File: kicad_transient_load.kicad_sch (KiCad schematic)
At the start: 6 parts, among them J1 BNC In, J2 Screw_Terminal_01x02, J3 Conn_02x03_Odd_Even

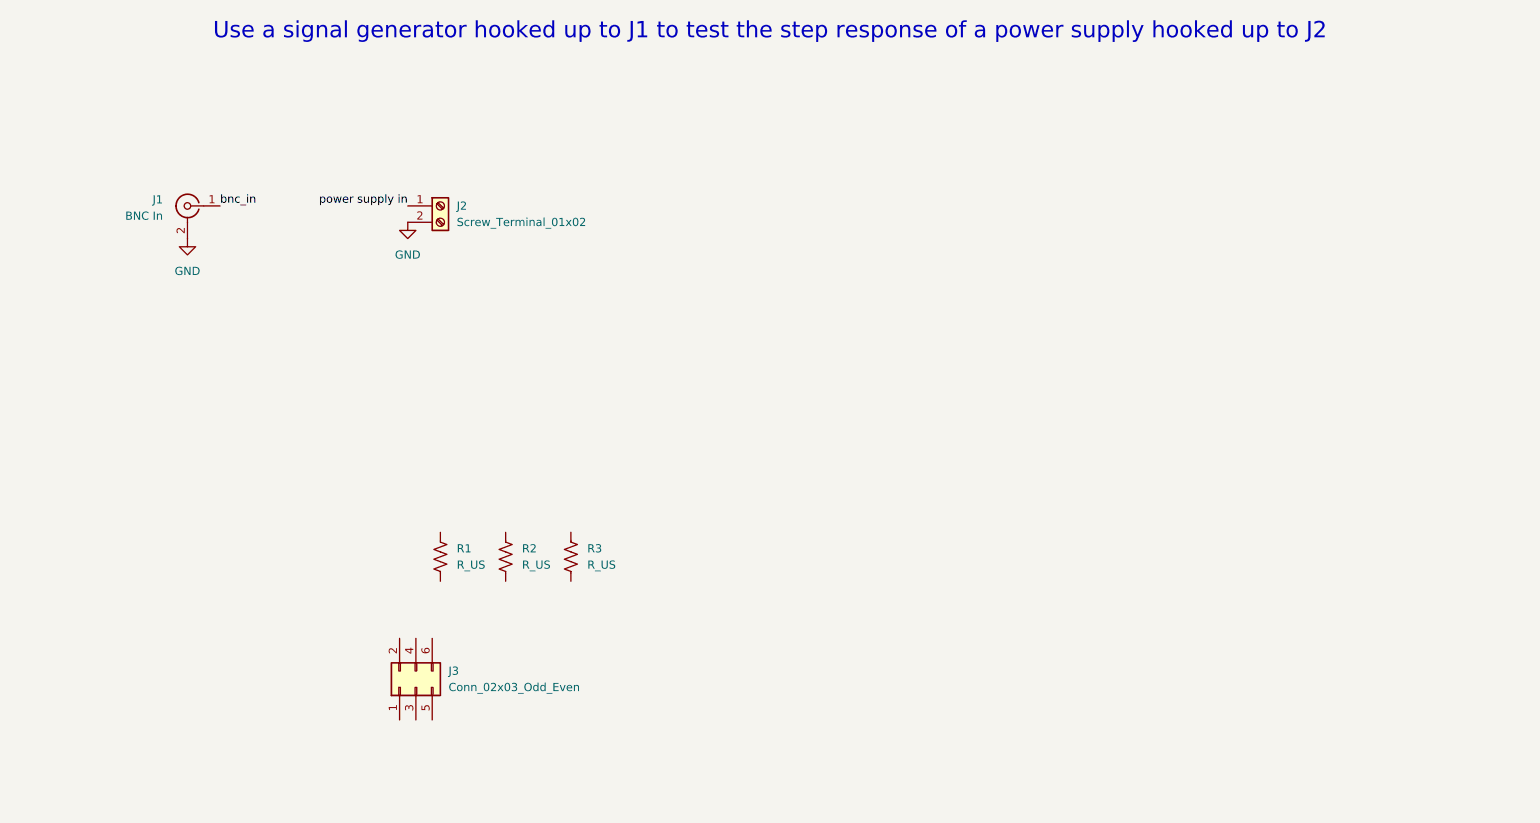
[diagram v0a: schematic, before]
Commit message: schematic laid out
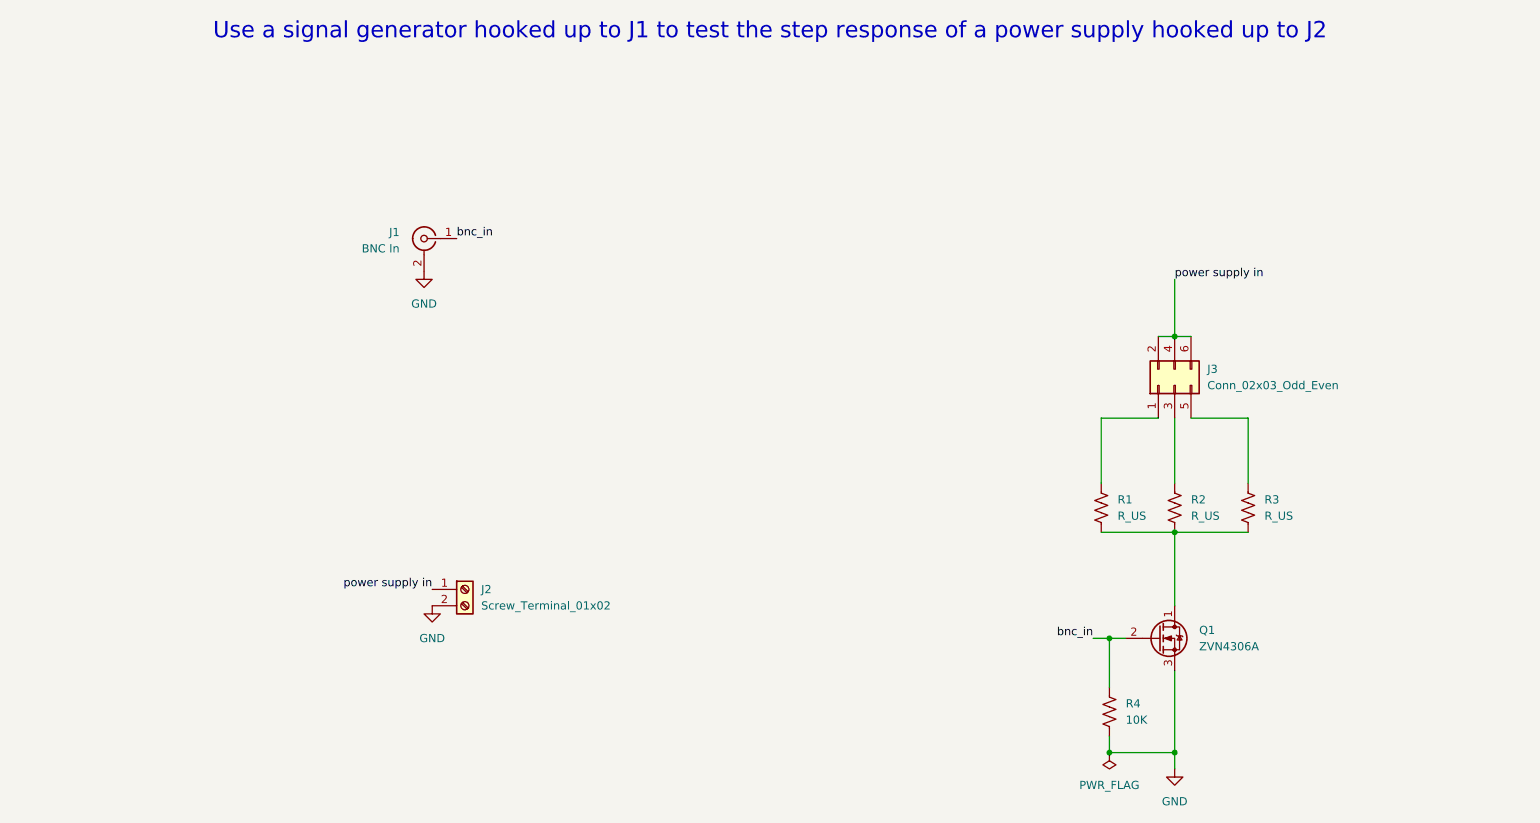
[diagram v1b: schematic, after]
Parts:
- added Q1: ZVN4306A, Package_TO_SOT_THT:TO-92_Inline, symbol Device:Q_NMOS_DGS
- added R4: 10K, symbol Device:R_US
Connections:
- net GND: now also Q1.3 (S), R4.1
- net bnc_in: now also Q1.2 (G), R4.2
- net power supply in: now also J3.2 (Pin_2), J3.4 (Pin_4), J3.6 (Pin_6)
- net at R3.1: now also J3.5 (Pin_5)
- net at R3.2: now also R1.2, R2.2, Q1.1 (D)
- net at R1.1: now also J3.1 (Pin_1)
- net at J3.3 (Pin_3): now also R2.1
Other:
- moved on the sheet: J1, J2, J3, R1, R2, R3

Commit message: Working on BNC footprint
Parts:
- J2: footprint (none) -> TerminalBlock_TE-Connectivity:TerminalBlock_TE_282834-2_1x02_P2.54mm_Horizontal; MFR (none) -> TE Connectivity; MFR Part No (none) -> 282834-2
- J3: footprint (none) -> Connector_PinHeader_2.54mm:PinHeader_2x03_P2.54mm_Vertical
- R1, R2, R3: footprint (none) -> Resistor_THT:R_Axial_DIN0918_L18.0mm_D9.0mm_P22.86mm_Horizontal; MFR (none) -> KOA Speer
- R4: footprint (none) -> Resistor_THT:R_Axial_DIN0207_L6.3mm_D2.5mm_P7.62mm_Horizontal; MFR (none) -> KOA Speer; MFR Part No (none) -> MF1/4LCT52R103J
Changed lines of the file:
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@@
 			)
 		)
-		(property "Footprint" ""
+		(property "Footprint" "Resistor_THT:R_Axial_DIN0918_L18.0mm_D9.0mm_P22.86mm_Horizontal"
 			(at 196.596 95.504 90)
 			(effects
@@
 			)
 		)
+		(property "MFR" "KOA Speer"
+			(at 195.58 95.25 0)
+			(effects
+				(font
+					(size 1.27 1.27)
+				)
+				(hide yes)
+			)
+		)
 		(pin "1"
 		)
@@
 			)
 		)
-		(property "Footprint" ""
+		(property "Footprint" "Resistor_THT:R_Axial_DIN0918_L18.0mm_D9.0mm_P22.86mm_Horizontal"
 			(at 173.736 95.504 90)
 			(effects
@@
 			)
 		)
+		(property "MFR" "KOA Speer"
+			(at 172.72 95.25 0)
+			(effects
+				(font
+					(size 1.27 1.27)
+				)
+				(hide yes)
+			)
+		)
 		(pin "1"
 		)
@@
 			)
 		)
-		(property "Footprint" ""
+		(property "Footprint" "Connector_PinHeader_2.54mm:PinHeader_2x03_P2.54mm_Vertical"
 			(at 184.15 76.2 0)
 			(effects
@@
 			)
 		)
+		(property "MFR" ""
+			(at 184.15 76.2 0)
+			(effects
+				(font
+					(size 1.27 1.27)
+				)
+				(hide yes)
+			)
+		)
+		(property "MFR Part No" ""
+			(at 184.15 76.2 0)
+			(effects
+				(font
+					(size 1.27 1.27)
+				)
+				(hide yes)
+			)
+		)
 		(pin "6"
 		)
@@
 			)
 		)
-		(property "Footprint" ""
+		(property "Footprint" "TerminalBlock_TE-Connectivity:TerminalBlock_TE_282834-2_1x02_P2.54mm_Horizontal"
 			(at 73.66 107.95 0)
 			(effects
@@
 			)
 		)
-		(property "MFR" ""
+		(property "MFR" "TE Connectivity"
 			(at 73.66 107.95 0)
 			(effects
@@
 			)
 		)
-		(property "MFR Part No" ""
+		(property "MFR Part No" "282834-2"
 			(at 73.66 107.95 0)
 			(effects
@@
 			)
 		)
-		(property "Footprint" ""
+		(property "Footprint" "Resistor_THT:R_Axial_DIN0918_L18.0mm_D9.0mm_P22.86mm_Horizontal"
 			(at 185.166 95.504 90)
 			(effects
@@
 			)
 		)
+		(property "MFR" "KOA Speer"
+			(at 184.15 95.25 0)
+			(effects
+				(font
+					(size 1.27 1.27)
+				)
+				(hide yes)
+			)
+		)
 		(pin "1"
 		)
@@
 			)
 		)
-		(property "Footprint" ""
+		(property "Footprint" "Resistor_THT:R_Axial_DIN0207_L6.3mm_D2.5mm_P7.62mm_Horizontal"
 			(at 172.974 126.746 90)
 			(effects
@@
 			(at 173.99 127 0)
 			(effects
+				(font
+					(size 1.27 1.27)
+				)
+				(hide yes)
+			)
+		)
+		(property "MFR" "KOA Speer"
+			(at 173.99 127 0)
+			(effects
+				(font
+					(size 1.27 1.27)
+				)
+				(hide yes)
+			)
+		)
+		(property "MFR Part No" "MF1/4LCT52R103J "
+			(at 173.99 127 0)
+			(effects

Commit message: finished footprint for BNC connector and added
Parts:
- J1: footprint (none) -> AAAA_Project_Library:BNC_TE-Connectivity_1-1337445-0
- J3: MFR (none) -> TE C onnectivity; MFR Part No (none) -> 9-146261-0
- R1, R2, R3: MFR KOA Speer -> (none)
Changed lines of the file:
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@@
 			)
 		)
-		(property "Footprint" ""
+		(property "Footprint" "AAAA_Project_Library:BNC_TE-Connectivity_1-1337445-0"
 			(at 67.31 53.34 0)
 			(effects
@@
 			)
 		)
-		(property "MFR" "KOA Speer"
+		(property "MFR" ""
 			(at 195.58 95.25 0)
 			(effects
@@
 			)
 		)
-		(property "MFR" "KOA Speer"
+		(property "MFR" ""
 			(at 172.72 95.25 0)
 			(effects
@@
 			)
 		)
-		(property "MFR" ""
+		(property "MFR" "TE C onnectivity"
 			(at 184.15 76.2 0)
 			(effects
@@
 			)
 		)
-		(property "MFR Part No" ""
+		(property "MFR Part No" "9-146261-0 "
 			(at 184.15 76.2 0)
 			(effects
@@
 			)
 		)
-		(property "MFR" "KOA Speer"
+		(property "MFR" ""
 			(at 184.15 95.25 0)
 			(effects
